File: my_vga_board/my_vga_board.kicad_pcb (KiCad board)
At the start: 4 copper layers, 85 x 56 mm, 71 parts, among them J1 AudioJack3, J2 AudioJack3, J3 Micro_SD_Card, J4 L77HDE15SD1CH4F, J5 USB_B_Micro, J6 Conn_01x02, J7 Conn_02x03_Odd_Even, SW1 SW_Push, SW2 SW_Push, SW3 SW_Push, SW4 SW_Push, U1 TLV70033_SOT23-5, U2 Pico, U3 NC7WZ16P6X, U4 PCM5101A

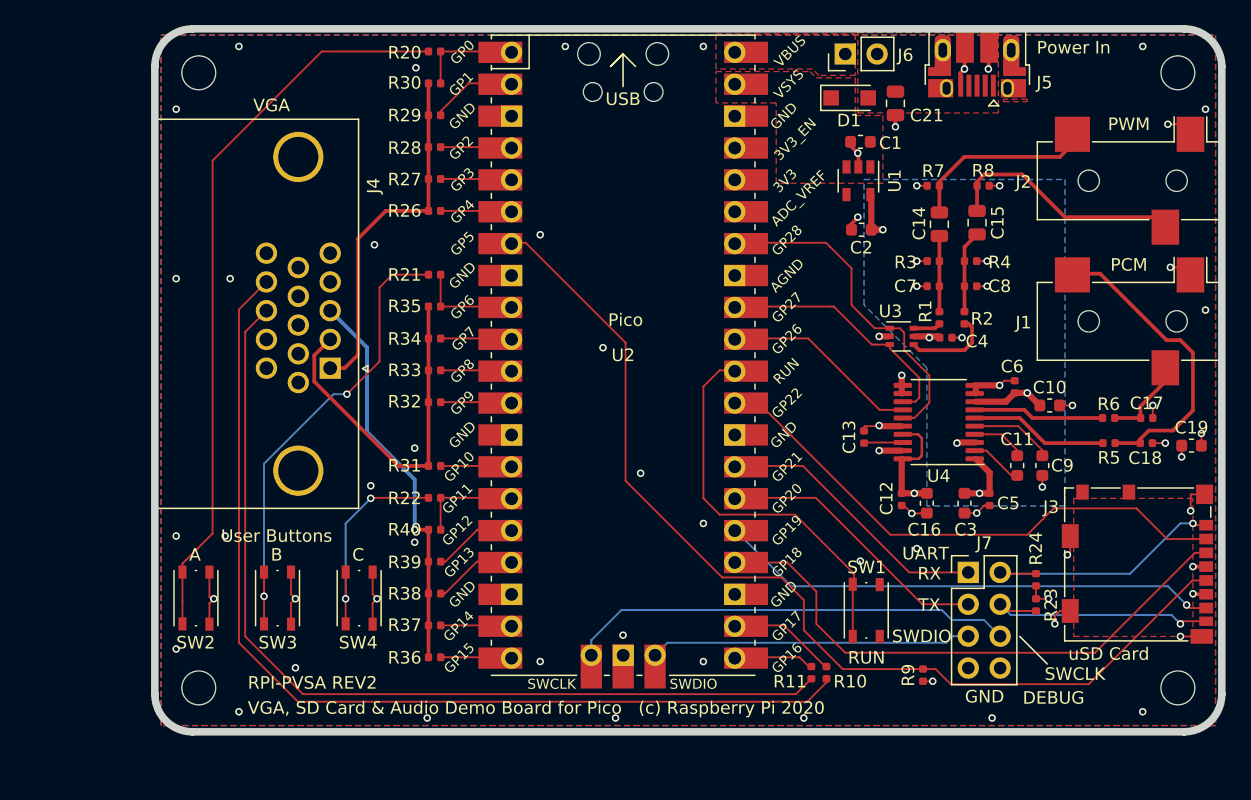
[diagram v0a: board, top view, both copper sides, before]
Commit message: updated commit
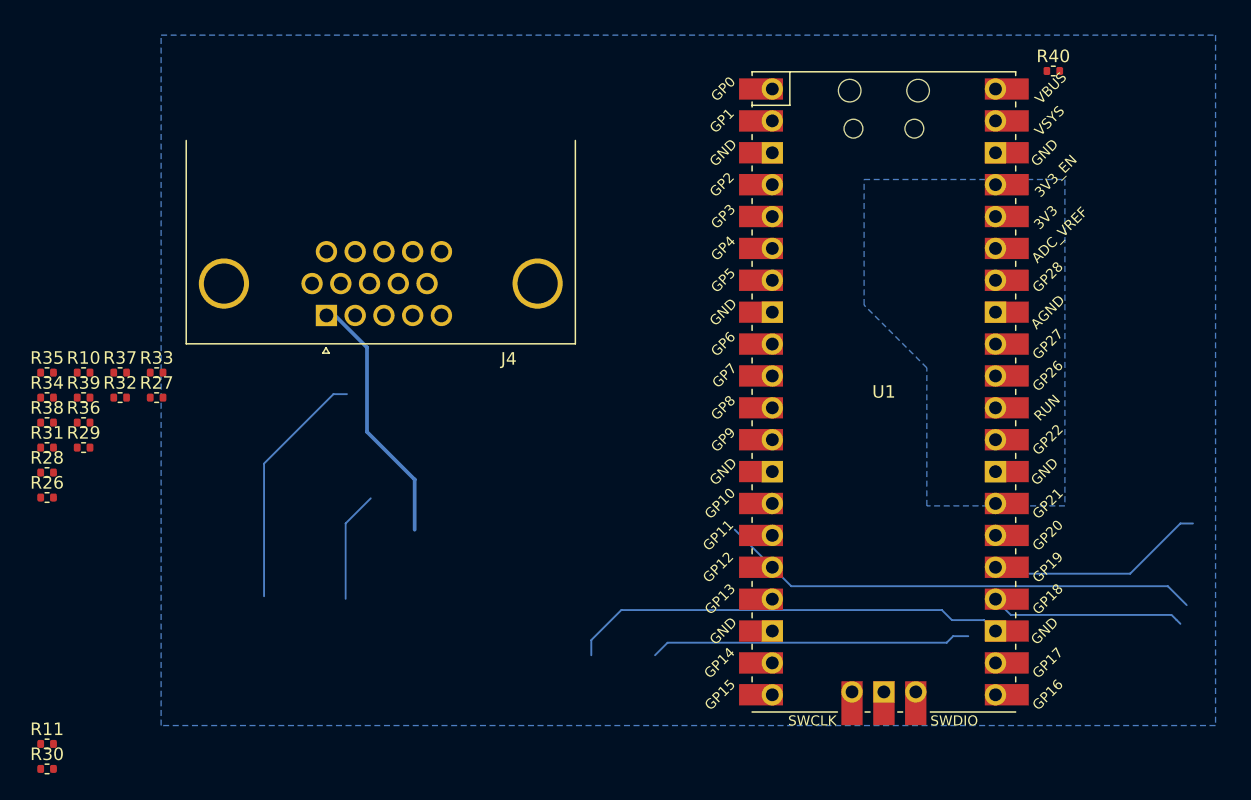
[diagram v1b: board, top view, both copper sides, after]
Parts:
- removed C1, C2: 1u, Capacitor_SMD:C_0603_1608Metric
- removed C10, C16, C19, C3: 10u, Capacitor_SMD:C_0603_1608Metric
- removed C11, C9: 2.2u, Capacitor_SMD:C_0603_1608Metric
- removed C12, C13, C4, C5, C6, C7, C8: 100n, Capacitor_SMD:C_0402_1005Metric
- removed C14, C15, C21: 47u, Capacitor_SMD:C_0805_2012Metric
- removed C17, C18: 2.2n, Capacitor_SMD:C_0402_1005Metric
- removed D1: MBR120, RPi_Pico:MBR120_SOD-123
- removed H1, H2, H3, H4: MountingHole, MountingHole:MountingHole_2.7mm_M2.5
- removed J1, J2: AudioJack3, RPi_Pico:CUI_SJ-3523-audio-jack
- removed J3: Micro_SD_Card, Connector_Card:microSD_HC_Molex_104031-0811
- removed J5: USB_B_Micro, RPi_Pico:USB_Micro-B_Amphenol_10103594-0001LF_Horizontal_modified
- removed J6: Conn_01x02, Connector_PinHeader_2.54mm:PinHeader_1x02_P2.54mm_Vertical
- removed J7: Conn_02x03_Odd_Even, Connector_PinHeader_2.54mm:PinHeader_2x04_P2.54mm_Vertical
- removed R1, R2: 220, Resistor_SMD:R_0402_1005Metric
- removed R20, R21, R22: 1k, Resistor_SMD:R_0402_1005Metric
- removed R23, R24: 10k, Resistor_SMD:R_0402_1005Metric
- removed R3, R4: 100, Resistor_SMD:R_0402_1005Metric
- removed R5, R6: 470, Resistor_SMD:R_0402_1005Metric
- removed R7, R8: 1.8K, Resistor_SMD:R_0402_1005Metric
- removed R9: DNF, Resistor_SMD:R_0402_1005Metric
- removed SW1, SW2, SW3, SW4: SW_Push, Button_Switch_SMD:SW_Push_1P1T_NO_Vertical_Wuerth_434133025816
- removed U2: Pico, RPi_Pico:RPi_Pico_SMD_TH
- removed U3: NC7WZ16P6X, Package_TO_SOT_SMD:SOT-363_SC-70-6
- removed U4: PCM5101A, Package_SO:TSSOP-20_4.4x6.5mm_P0.65mm
- U1: value TLV70033_SOT23-5 -> Pico; footprint Package_TO_SOT_SMD:SOT-23-5 -> RPi_Pico:RPi_Pico_SMD_TH
- moved R10 63.8 mm to (87.8, 76.4), turned to 0 degrees
- moved R30 62.7 mm to (84.9, 108.0)
- moved R40 61.4 mm to (165.1, 52.4)
- moved R11 61.1 mm to (84.9, 106.0), turned to 0 degrees
- moved R28 40.3 mm to (84.9, 84.3)
- moved R29 38.5 mm to (87.8, 82.4)
- moved R26 38.4 mm to (84.9, 86.3)
- moved R38 33.7 mm to (84.9, 80.4)
- moved R36 33.6 mm to (87.8, 80.4)
- moved R37 32.1 mm to (90.7, 76.4)
- moved R35 31.3 mm to (84.9, 76.4)
- moved R34 31.2 mm to (84.9, 78.4)
- moved R31 30.9 mm to (84.9, 82.4)
- moved R39 30.9 mm to (87.8, 78.4)
- moved R27 28.2 mm to (93.6, 78.4)
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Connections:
- J4 pad 11: Net-(J4-Pad11) -> unconnected-(J4-Pad11)
- J4 pad 12: Net-(J4-Pad12) -> unconnected-(J4-Pad12)
- J4 pad 15: Net-(J4-Pad15) -> unconnected-(J4-Pad15)
- J4 pad 4: Net-(J4-Pad4) -> unconnected-(J4-Pad4)
- J4 pad 9: Net-(J4-Pad9) -> unconnected-(J4-Pad9)
- U1 pad 1: /VSYS -> /GPIO0
- U1 pad 2: GND -> /GPIO1
- U1 pad 3: /VSYS -> GND
- U1 pad 4: Net-(U1-Pad4) -> /GPIO2
- U1 pad 5: +3.3VA -> /GPIO3
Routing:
- net (no net): track 0.00 -> 89.5 mm
- net /GPIO5: track 81.2 -> 0.00 mm
- net /VSYNC: track 79.3 -> 0.00 mm
- net /HSYNC: track 74.2 -> 0.00 mm
- net Net-(R20-Pad2): track 59.0 -> 0.00 mm
- net GND: track 53.9 -> 0.00 mm, vias 66 -> 0
- net /GPIO18: track 46.9 -> 0.00 mm
- net /GPIO22: track 43.8 -> 0.00 mm
- net /GPIO19: track 40.1 -> 0.00 mm, vias 1 -> 0
- net Net-(R21-Pad2): track 37.5 -> 0.00 mm, vias 2 -> 0
- net /SWCLK: track 35.6 -> 0.00 mm
- net /GPIO12: track 6.59 -> 38.5 mm
- net /VGA_B: track 31.5 -> 0.00 mm, vias 1 -> 0
- net /RUN: track 31.5 -> 0.00 mm
- net /VGA_G: track 28.8 -> 0.00 mm
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- added copper zone on B.Cu, net (none)
- removed copper zone on B.Cu, net +3.3VA
- removed copper zone on B.Cu, net +3V3
- removed copper zone on F.Cu, net +5V
- removed copper zone on F.Cu, net /VSYS
- removed copper zone on F.Cu, net GND
- removed copper zone on F.Cu, net VBUS
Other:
- board outline removed
- net class Default removed
- board text removed: "A"
- board text removed: "B"
- board text removed: "C"
- board text removed: "DEBUG"
- board text removed: "GND"
- board text removed: "PCM"
- board text removed: "PWM"
- board text removed: "Pico"
- board text removed: "Power In"
- board text removed: "RPI-PVSA REV2"
- board text removed: "RUN"
- board text removed: "RX"
- board text removed: "SWCLK"
- board text removed: "SWDIO"
- board text removed: "TX"
- board text removed: "UART"
- board text removed: "USB"
- board text removed: "User Buttons"
- board text removed: "VGA"
- board text removed: "VGA, SD Card & Audio Demo Board for Pico (c) Raspberry Pi 2020"
- board text removed: "uSD Card"
